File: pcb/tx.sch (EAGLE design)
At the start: 51 parts, among them U3 MCP73831T-2ACI/OT, Y1 CRYSTAL-26MHZSMD-3.2X2.5

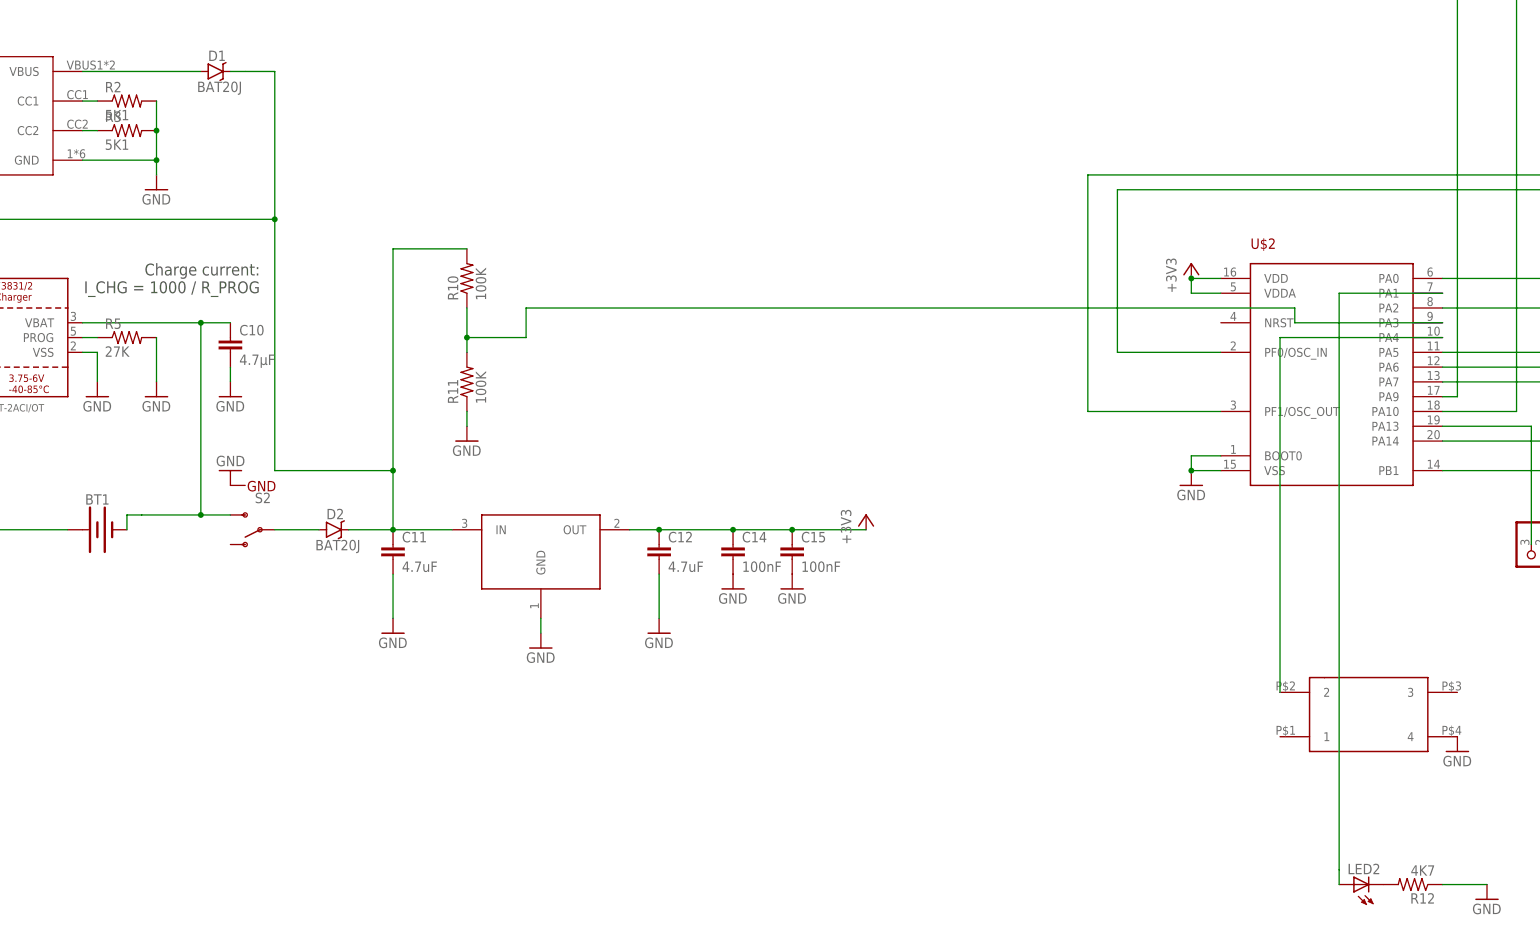
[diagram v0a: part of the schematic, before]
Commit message: cleanup
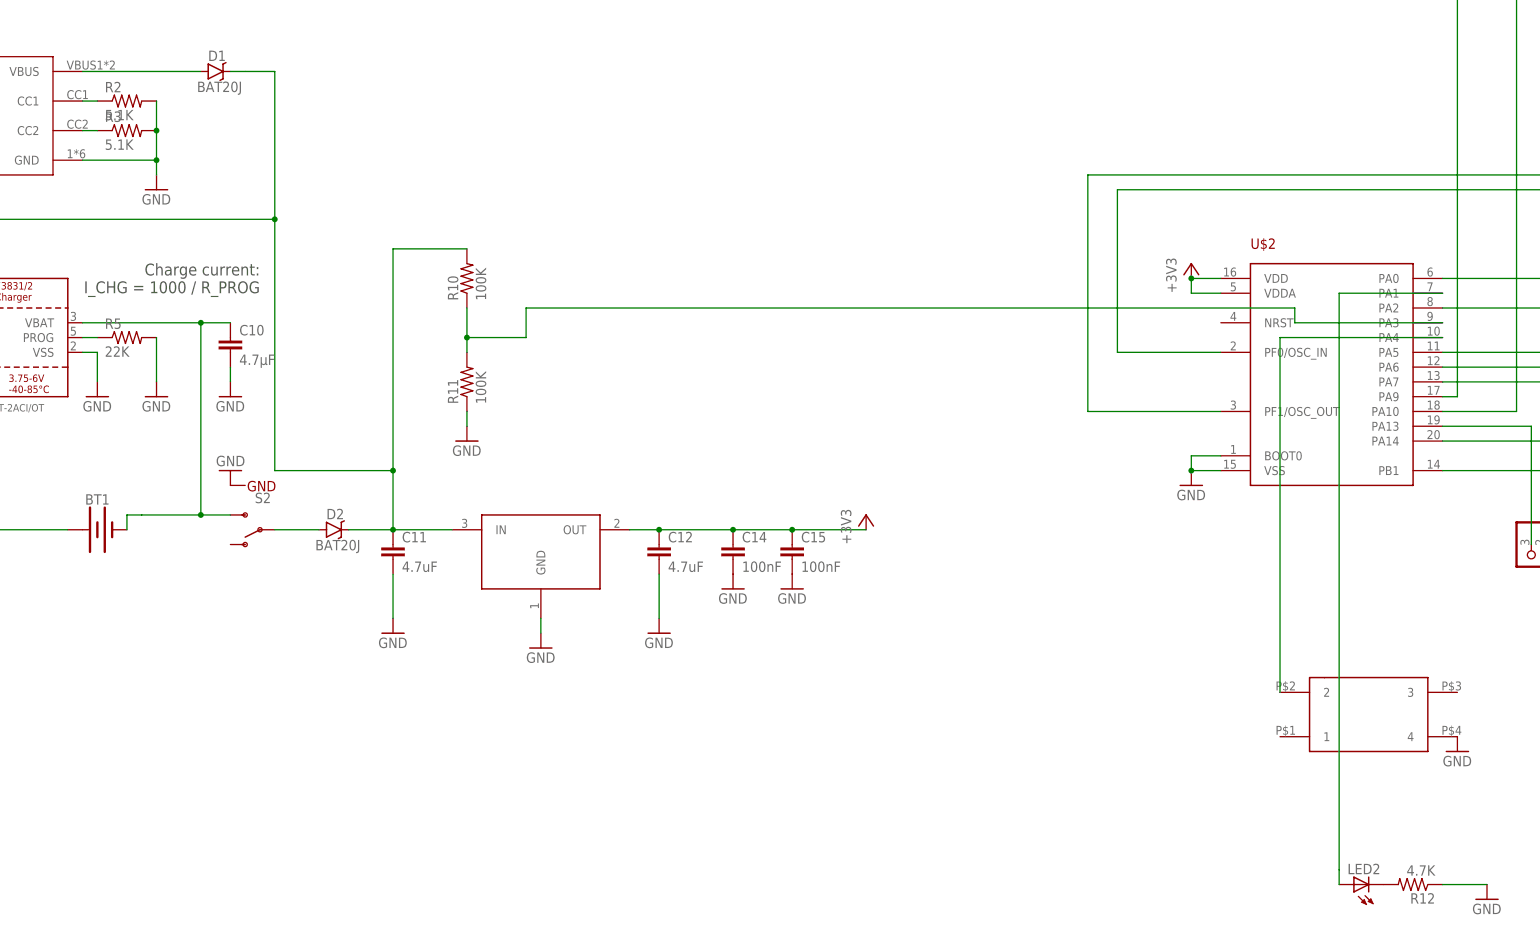
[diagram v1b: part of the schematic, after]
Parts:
- R12: value 4K7 -> 4.7K
- R2, R3: value 5K1 -> 5.1K
- R5: value 27K -> 22K
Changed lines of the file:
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@@
 <part name="Y1" library="SparkFun-Clocks" deviceset="CRYSTAL-26MHZ" device="SMD-3.2X2.5"/>
 <part name="GND6" library="supply1" deviceset="GND" device=""/>
-<part name="R3" library="joyAnalog" deviceset="RESISTOR" device="0805-RES" value="5K1"/>
-<part name="R2" library="joyAnalog" deviceset="RESISTOR" device="0805-RES" value="5K1"/>
+<part name="R3" library="joyAnalog" deviceset="RESISTOR" device="0805-RES" value="5.1K"/>
+<part name="R2" library="joyAnalog" deviceset="RESISTOR" device="0805-RES" value="5.1K"/>
 <part name="U3" library="microbuilder" deviceset="MCP73831/2" device="" value="MCP73831T-2ACI/OT"/>
 <part name="R4" library="SparkFun-Passives" deviceset="RESISTOR" device="0805-RES" value="4.7K"/>
 <part name="C10" library="SparkFun-Passives" deviceset="CAP" device="0805" value="4.7µF"/>
-<part name="R5" library="SparkFun-Passives" deviceset="RESISTOR" device="0805-RES" value="27K"/>
+<part name="R5" library="SparkFun-Passives" deviceset="RESISTOR" device="0805-RES" value="22K"/>
 <part name="GND7" library="supply1" library_urn="urn:adsk.eagle:library:371" deviceset="GND" device=""/>
 <part name="U$9" library="3pos_slide_switch" deviceset="XC6206_DEV" device=""/>
@@
 <part name="GND26" library="clock" deviceset="GND" device=""/>
 <part name="LED2" library="joyAnalog" deviceset="LED" device="CHIP-LED0805"/>
-<part name="R12" library="joyAnalog" deviceset="RESISTOR" device="0805-RES" value="4K7"/>
+<part name="R12" library="joyAnalog" deviceset="RESISTOR" device="0805-RES" value="4.7K"/>
 <part name="GND27" library="supply1" library_urn="urn:adsk.eagle:library:371" deviceset="GND" device=""/>
 <part name="GND28" library="supply1" library_urn="urn:adsk.eagle:library:371" deviceset="GND" device=""/>
